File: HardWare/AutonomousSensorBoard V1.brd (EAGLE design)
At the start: 100 x 100 mm, 10 parts

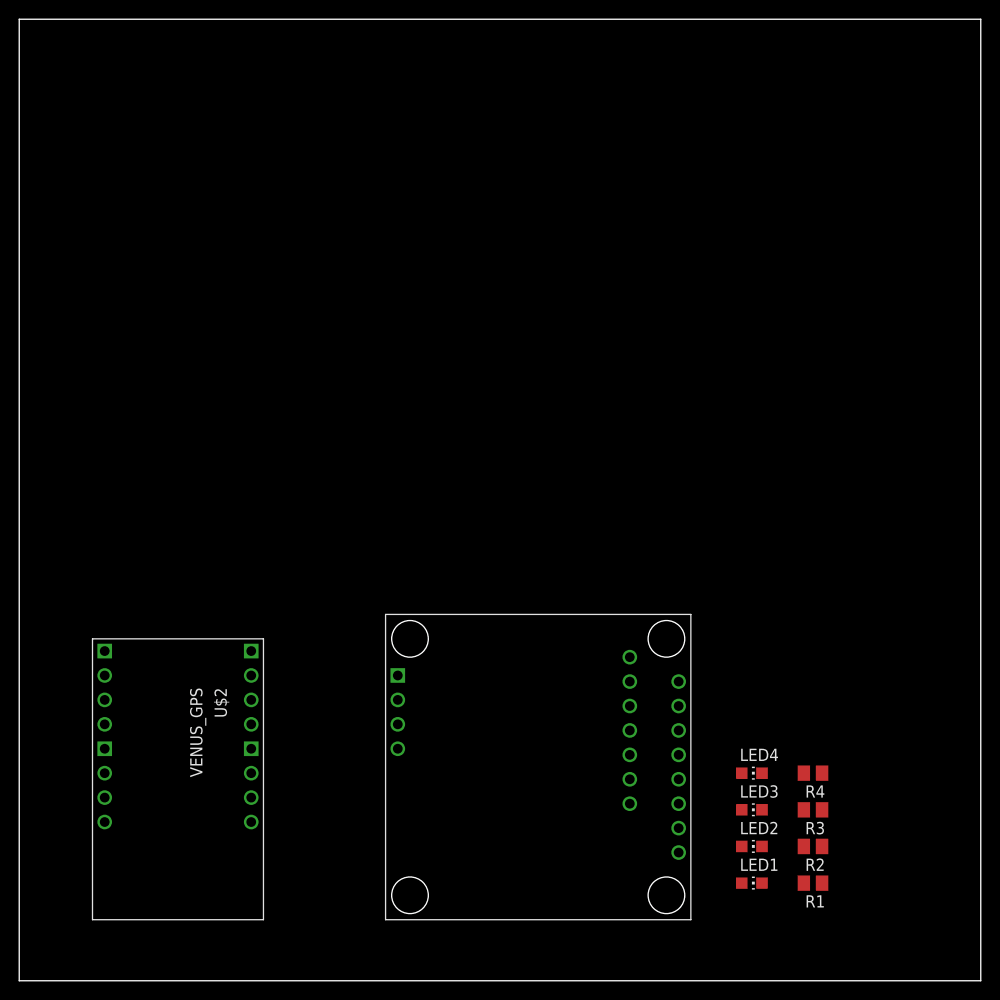
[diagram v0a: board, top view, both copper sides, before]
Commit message: gerbers generated
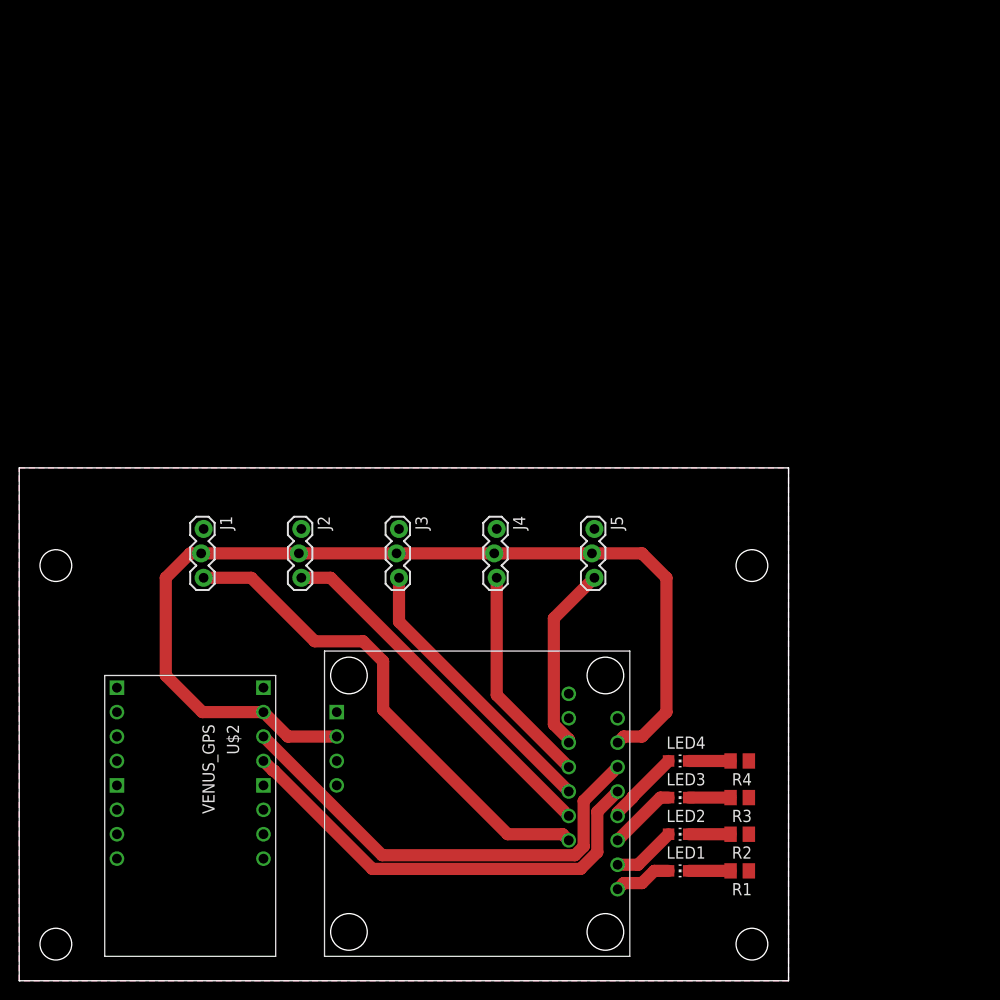
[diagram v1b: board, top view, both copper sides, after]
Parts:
- added FRAME1: FRAME-LEDGER, SparkFun-Aesthetics:CREATIVE_COMMONS
- added H1, H2, H3, H4: STAND-OFF, SparkFun-Electromechanical:STAND-OFF
- added J1, J2, J3, J4, J5: (no value), SparkFun-Connectors:1X03_LOCK
- moved LED1 7.73 mm to (68.6, 11.4)
- moved LED2 7.73 mm to (68.6, 15.2)
- moved LED3 7.73 mm to (68.6, 19.1)
- moved LED4 7.73 mm to (68.6, 22.9)
- moved R1 7.73 mm to (74.9, 11.4)
- moved R2 7.73 mm to (74.9, 15.2)
- moved R3 7.73 mm to (74.9, 19.1)
- moved R4 7.73 mm to (74.9, 22.9)
- moved U$1 7.41 mm to (31.8, 2.54)
- moved U$2 4.02 mm to (8.89, 31.8)
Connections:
- new net A0: J1.3, U$1.A0
- new net A1: J2.3, U$1.A1
- new net A2: J3.3, U$1.A2
- new net A3: J4.3, U$1.A3
- new net A4: J5.3, U$1.A4
- net 3.3V: now also J1.2, J2.2, J3.2, J4.2, J5.2
- net GND: now also J1.1, J2.1, J3.1, J4.1, J5.1
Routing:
- net 3.3V: track 0.00 -> 105.1 mm
- net A0: track 0.00 -> 52.2 mm
- net N$1: track 0.00 -> 48.5 mm
- net N$2: track 0.00 -> 47.3 mm
- net A1: track 0.00 -> 38.1 mm
- net A2: track 0.00 -> 29.5 mm
- net A3: track 0.00 -> 22.8 mm
- net A4: track 0.00 -> 19.5 mm
- net N$10: track 0.00 -> 7.91 mm
- net N$9: track 0.00 -> 7.14 mm
- net N$7: track 0.00 -> 6.62 mm
- net N$8: track 0.00 -> 6.09 mm
- net N$6: track 0.00 -> 4.35 mm
- net N$5: track 0.00 -> 4.35 mm
- net N$4: track 0.00 -> 4.35 mm
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- added copper zone on layer 1, net GND
- added copper zone on layer 16, net GND
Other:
- board size 100 x 100 mm -> 80 x 53.3 mm
